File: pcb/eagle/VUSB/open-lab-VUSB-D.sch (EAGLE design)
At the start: 72 parts, among them IC1 ATMEGA328P, IC2 MCP73831, IC4 MCP1700-33, IC5 MCP23008, IC6 MAX31855, IC7 ENC28J60, J1 AYZ0202, Q1 BSS123, Q2 BSS123, Q3 BSS123, X1 USBSMD, X2 32.768kHz, X3 25MHz

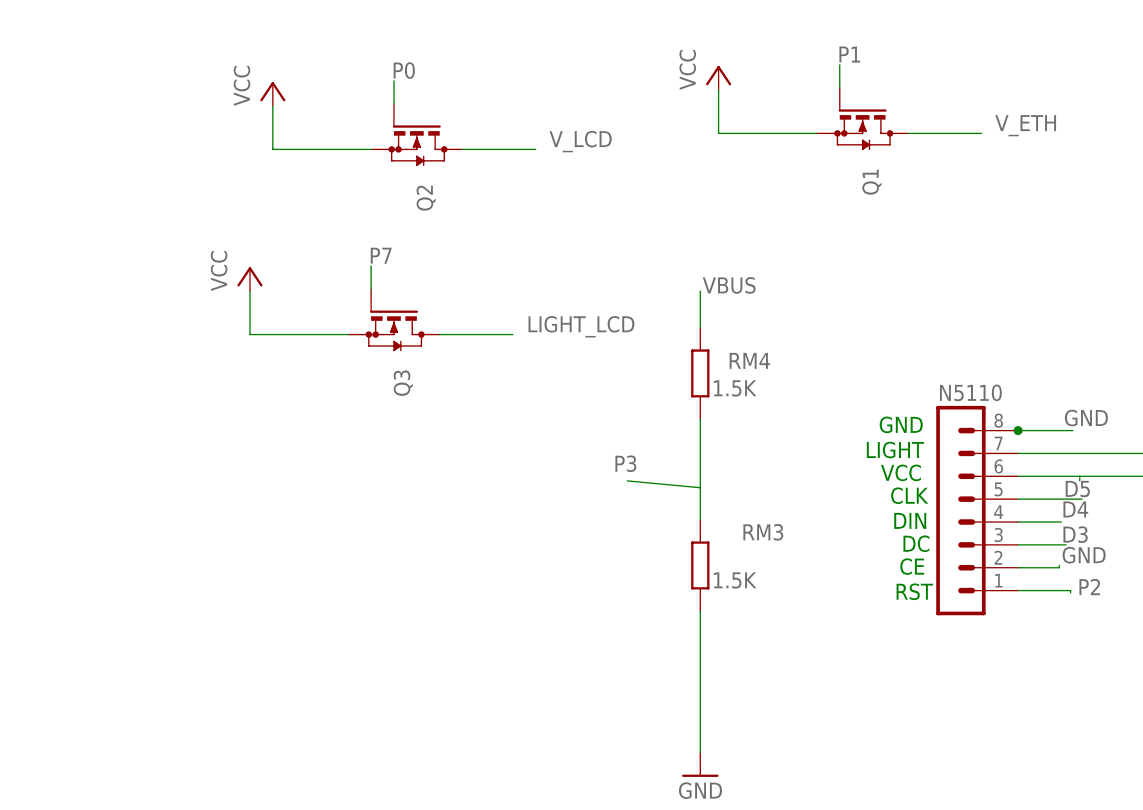
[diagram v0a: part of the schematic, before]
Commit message: update
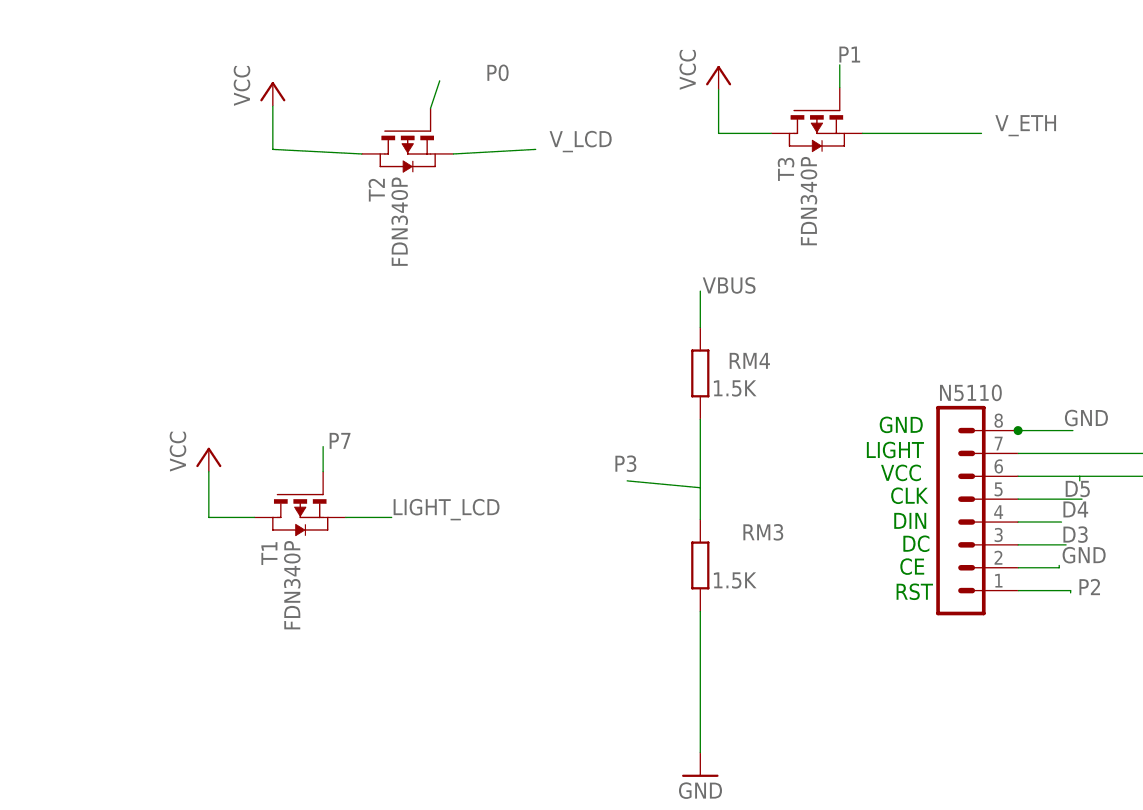
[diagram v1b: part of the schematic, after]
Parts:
- removed Q1, Q2, Q3: BSS123, transistor-small-signal:BSS123
- added T1, T2, T3: FDN340P, zetex:PMOSSOT23
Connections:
- net LIGHT_LCD: now also T1.S; no longer Q3.D
- net P0: now also T2.G; no longer Q2.G
- net P1: now also T3.G; no longer Q1.G
- net P7: now also T1.G; no longer Q3.G
- net VCC: now also T1.D, T2.D, T3.D; no longer Q1.S, Q2.S, Q3.S
- net V_ETH: now also T3.S; no longer Q1.D
- net V_LCD: now also T2.S; no longer Q2.D
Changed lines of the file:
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@@
 </variantdefs>
 <classes>
-<class number="0" name="default" width="0.2032" drill="0">
+<class number="0" name="default" width="0.254" drill="0">
+<clearance class="0" value="0.254"/>
 </class>
 <class number="1" name="power" width="0.381" drill="0">
+</class>
+<class number="3" name="usbvcc" width="0.508" drill="0.6096">
+<clearance class="3" value="0.254"/>
 </class>
 </classes>
@@
 <part name="C6" library="resistor" deviceset="C-EU" device="C0805" value=".1u"/>
 <part name="P+17" library="supply1" deviceset="VCC" device=""/>
-<part name="Q1" library="transistor-small-signal" deviceset="BSS123" device=""/>
 <part name="P+7" library="supply1" deviceset="VCC" device=""/>
-<part name="Q2" library="transistor-small-signal" deviceset="BSS123" device=""/>
 <part name="P+8" library="supply1" deviceset="VCC" device=""/>
 <part name="IC5" library="JeeLabs" deviceset="MCP23008" device="T" value="MCP23008"/>
@@
 <part name="P+16" library="supply1" deviceset="VCC" device=""/>
 <part name="SUPPLY2" library="supply2" deviceset="GND" device=""/>
-<part name="Q3" library="transistor-small-signal" deviceset="BSS123" device=""/>
-<part name="P+19" library="supply1" deviceset="VCC" device=""/>
 <part name="GND12" library="supply1" deviceset="GND" device=""/>
 <part name="BTN1" library="adafruit" deviceset="EVQQ2" device="" value=""/>
@@
 <part name="SV2" library="con-lstb" deviceset="MA06-2" device=""/>
 <part name="SV1" library="con-lstb" deviceset="MA04-1" device=""/>
+<part name="T1" library="zetex" deviceset="PMOSSOT23" device="" value="FDN340P"/>
+<part name="P+3" library="supply1" deviceset="VCC" device=""/>
+<part name="T2" library="zetex" deviceset="PMOSSOT23" device="" value="FDN340P"/>
+<part name="T3" library="zetex" deviceset="PMOSSOT23" device="" value="FDN340P"/>
 </parts>
 <sheets>
@@
 </instance>
 <instance part="P+17" gate="VCC" x="308.102" y="4.572"/>
-<instance part="Q1" gate="G$1" x="219.964" y="167.132" smashed="yes" rot="R270">
-<attribute name="NAME" x="219.964" y="163.322" size="1.778" layer="95" rot="R270"/>
-</instance>
 <instance part="P+7" gate="VCC" x="203.962" y="174.498"/>
-<instance part="Q2" gate="G$1" x="170.434" y="165.354" smashed="yes" rot="R270">
-<attribute name="NAME" x="170.434" y="161.544" size="1.778" layer="95" rot="R270"/>
-</instance>
 <instance part="P+8" gate="VCC" x="154.432" y="172.72"/>
 <instance part="IC5" gate="G$1" x="-15.24" y="-53.34"/>
@@
 <instance part="P+16" gate="VCC" x="-42.418" y="-28.194"/>
 <instance part="SUPPLY2" gate="GND" x="-36.83" y="-82.042"/>
-<instance part="Q3" gate="G$1" x="167.894" y="144.78" smashed="yes" rot="R270">
-<attribute name="NAME" x="167.894" y="140.97" size="1.778" layer="95" rot="R270"/>
-</instance>
-<instance part="P+19" gate="VCC" x="151.892" y="152.146"/>
 <instance part="GND12" gate="1" x="171.45" y="21.844"/>
 <instance part="BTN1" gate="G$1" x="176.53" y="26.924" rot="R270"/>
@@
 <instance part="SV2" gate="1" x="51.054" y="-53.34"/>
 <instance part="SV1" gate="1" x="236.728" y="52.832"/>
+<instance part="T1" gate="A" x="157.48" y="124.46" rot="MR270"/>
+<instance part="P+3" gate="VCC" x="147.32" y="132.08"/>
+<instance part="T2" gate="A" x="169.418" y="164.846" rot="MR270"/>
+<instance part="T3" gate="A" x="214.884" y="167.132" rot="MR270"/>
 </instances>
 <busses>
@@
 </segment>
 <segment>
-<pinref part="Q1" gate="G$1" pin="S"/>
-<wire x1="214.884" y1="167.132" x2="203.962" y2="167.132" width="0.1524" layer="91"/>
+<wire x1="209.804" y1="167.132" x2="203.962" y2="167.132" width="0.1524" layer="91"/>
 <wire x1="203.962" y1="167.132" x2="203.962" y2="171.958" width="0.1524" layer="91"/>
 <pinref part="P+7" gate="VCC" pin="VCC"/>
-</segment>
-<segment>
-<pinref part="Q2" gate="G$1" pin="S"/>
-<wire x1="165.354" y1="165.354" x2="154.432" y2="165.354" width="0.1524" layer="91"/>
+<pinref part="T3" gate="A" pin="D"/>
+</segment>
+<segment>
+<wire x1="164.338" y1="164.846" x2="154.432" y2="165.354" width="0.1524" layer="91"/>
 <wire x1="154.432" y1="165.354" x2="154.432" y2="170.18" width="0.1524" layer="91"/>
 <pinref part="P+8" gate="VCC" pin="VCC"/>
+<pinref part="T2" gate="A" pin="D"/>
 </segment>
 <segment>
@@
 </segment>
 <segment>
-<pinref part="Q3" gate="G$1" pin="S"/>
-<wire x1="162.814" y1="144.78" x2="151.892" y2="144.78" width="0.1524" layer="91"/>
-<wire x1="151.892" y1="144.78" x2="151.892" y2="149.606" width="0.1524" layer="91"/>
-<pinref part="P+19" gate="VCC" pin="VCC"/>
-</segment>
-<segment>
 <wire x1="43.434" y1="-50.8" x2="41.91" y2="-50.8" width="0.1524" layer="91"/>
 <label x="34.036" y="-50.8" size="1.778" layer="95"/>
 <pinref part="SV2" gate="1" pin="10"/>
+</segment>
+<segment>
+<pinref part="T1" gate="A" pin="D"/>
+<wire x1="152.4" y1="124.46" x2="147.32" y2="124.46" width="0.1524" layer="91"/>
+<wire x1="147.32" y1="124.46" x2="147.32" y2="129.54" width="0.1524" layer="91"/>
+<pinref part="P+3" gate="VCC" pin="VCC"/>
 </segment>
 </net>
@@
 </segment>
 <segment>
-<pinref part="Q1" gate="G$1" pin="D"/>
-<wire x1="225.044" y1="167.132" x2="233.172" y2="167.132" width="0.1524" layer="91"/>
+<wire x1="219.964" y1="167.132" x2="233.172" y2="167.132" width="0.1524" layer="91"/>
 <label x="234.696" y="167.386" size="1.778" layer="95"/>
+<pinref part="T3" gate="A" pin="S"/>
 </segment>
 </net>
 <net name="V_LCD" class="0">
 <segment>
-<pinref part="Q2" gate="G$1" pin="D"/>
-<wire x1="175.514" y1="165.354" x2="183.642" y2="165.354" width="0.1524" layer="91"/>
+<wire x1="174.498" y1="164.846" x2="183.642" y2="165.354" width="0.1524" layer="91"/>
 <label x="185.166" y="165.608" size="1.778" layer="95"/>
+<pinref part="T2" gate="A" pin="S"/>
 </segment>
 <segment>
@@
 </segment>
 <segment>
-<pinref part="Q3" gate="G$1" pin="D"/>
-<wire x1="172.974" y1="144.78" x2="181.102" y2="144.78" width="0.1524" layer="91"/>
-<label x="182.626" y="145.034" size="1.778" layer="95"/>
+<pinref part="T1" gate="A" pin="S"/>
+<wire x1="162.56" y1="124.46" x2="167.64" y2="124.46" width="0.1524" layer="91"/>
+<label x="167.64" y="124.714" size="1.778" layer="95"/>
 </segment>
 </net>
@@
 </segment>
 <segment>
-<pinref part="Q3" gate="G$1" pin="G"/>
-<wire x1="165.354" y1="149.86" x2="165.354" y2="152.4" width="0.1524" layer="91"/>
-<label x="165.1" y="152.654" size="1.778" layer="95"/>
+<pinref part="T1" gate="A" pin="G"/>
+<wire x1="160.02" y1="129.54" x2="160.02" y2="132.334" width="0.1524" layer="91"/>
+<label x="160.528" y="132.08" size="1.778" layer="95"/>
 </segment>
 </net>
@@
 </segment>
 <segment>
-<pinref part="Q1" gate="G$1" pin="G"/>
 <wire x1="217.424" y1="172.212" x2="217.424" y2="174.752" width="0.1524" layer="91"/>
 <label x="217.17" y="175.006" size="1.778" layer="95"/>
+<pinref part="T3" gate="A" pin="G"/>
 </segment>
 </net>
@@
 </segment>
 <segment>
-<pinref part="Q2" gate="G$1" pin="G"/>
-<wire x1="167.894" y1="170.434" x2="167.894" y2="172.974" width="0.1524" layer="91"/>
-<label x="167.64" y="173.228" size="1.778" layer="95"/>
-</segment>
-</net>
+<label x="178.054" y="172.974" size="1.778" layer="95"/>
+<pinref part="T2" gate="A" pin="G"/>
+<wire x1="171.958" y1="169.926" x2="172.974" y2="172.974" width="0.1524" layer="91"/>
+</segment>
+</net>
